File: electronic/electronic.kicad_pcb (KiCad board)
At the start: 2 copper layers, 64.5 x 63 mm, 16 parts, among them J1 M_PWM, J10 BMP01, J11 MPU6050_01, J12 NEO_06_01, J14 OLED, J15 HCSR01, J16 HCSR02, J17 HCSR03, J18 HCSR04, J2 BAT_AX, J20 25.5-24 ESP32, U10 DEVKIT_V1_ESP32-WROOM-32, U6 DHT22

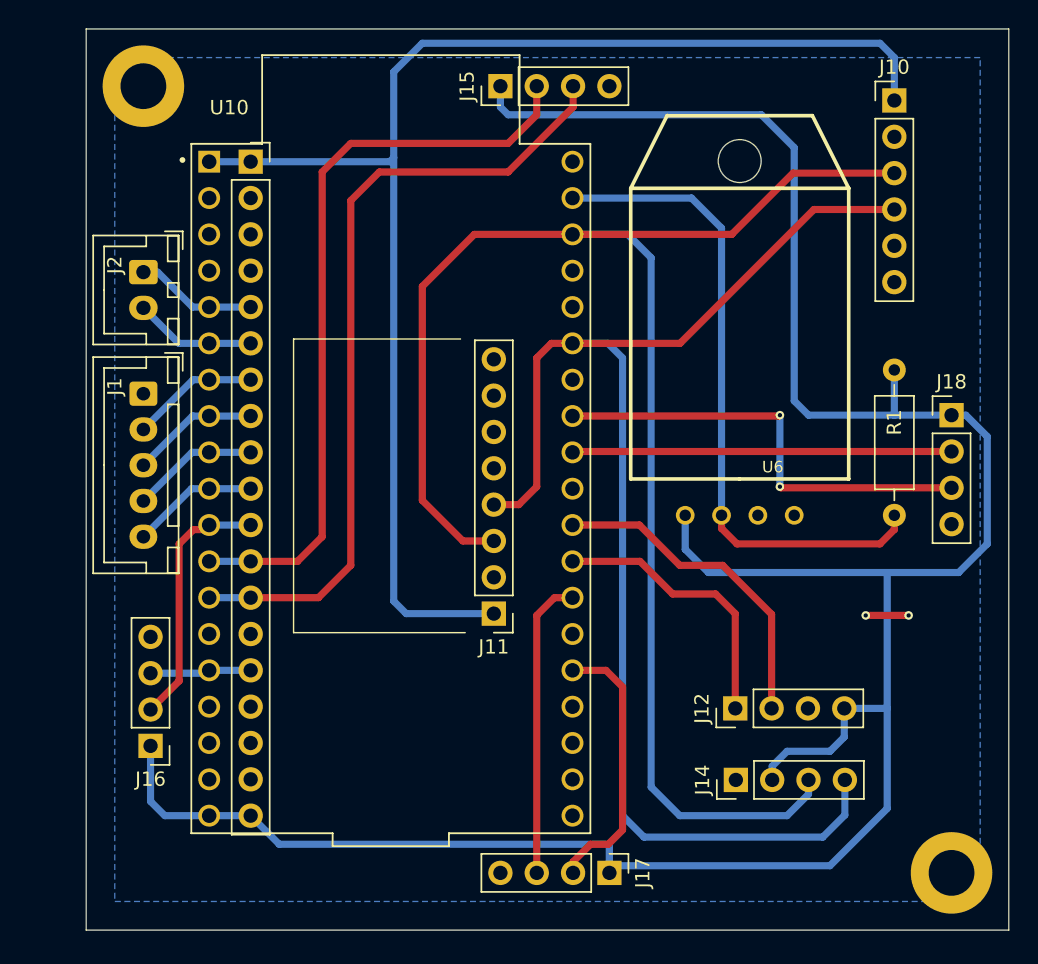
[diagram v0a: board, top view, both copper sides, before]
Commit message: chore (electronic | power): update electronic subprojects
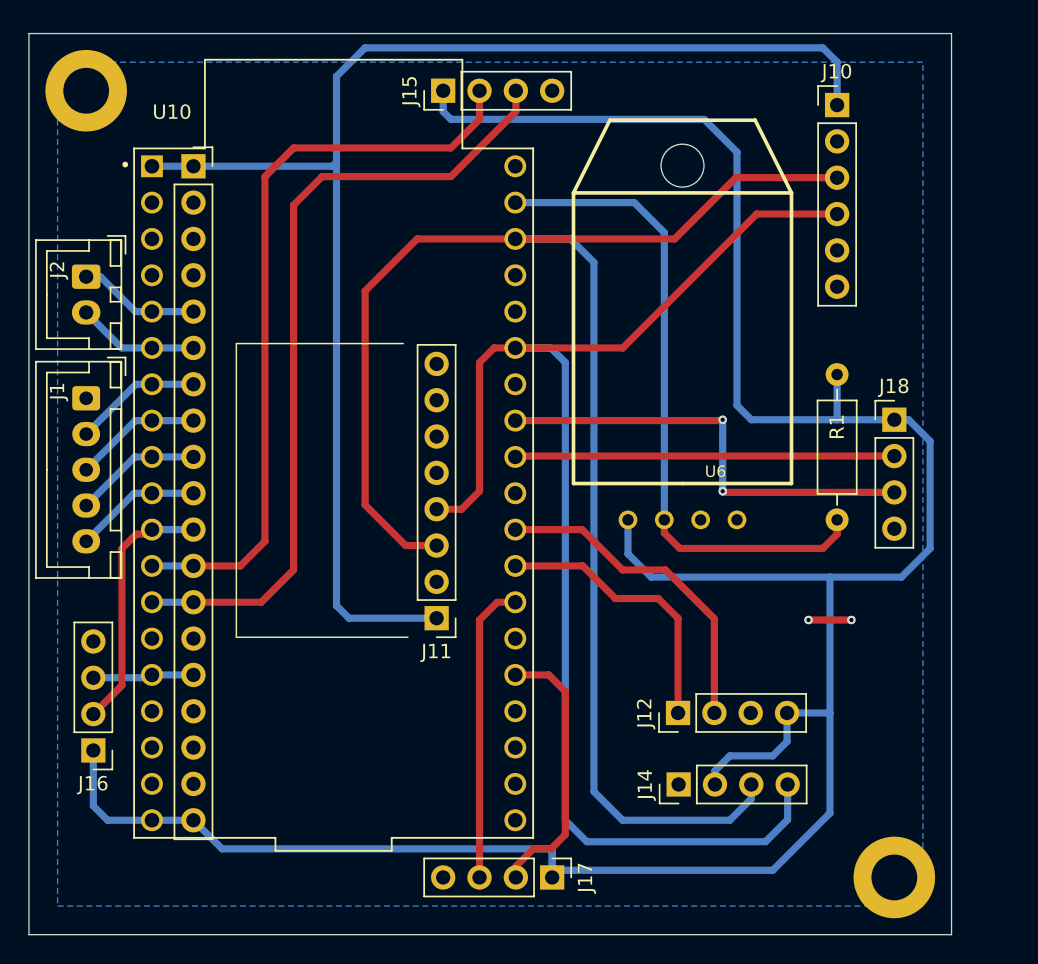
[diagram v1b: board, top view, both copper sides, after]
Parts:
- moved J1 4.01 mm to (18.5, 39.8)
- moved J10 4.01 mm to (71.0, 19.3)
- moved J11 4.01 mm to (43.0, 55.2)
- moved J12 4.01 mm to (59.9, 61.8)
- moved J15 4.01 mm to (43.5, 18.3)
- moved J18 4.01 mm to (75.0, 41.3)
- moved J2 4.01 mm to (18.5, 31.3)
- moved J20 4.01 mm to (26.0, 23.6)
- moved REF** 4.01 mm to (18.5, 18.3)
- moved U10 4.01 mm to (35.8, 46.5)
- moved U6 4.01 mm to (60.2, 48.3)
- moved J14 4.01 mm to (59.9, 66.8)
- moved J16 4.01 mm to (19.0, 64.4)
- moved J17 4.01 mm to (51.1, 73.3)
- moved R1 4.01 mm to (71.0, 38.2)
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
